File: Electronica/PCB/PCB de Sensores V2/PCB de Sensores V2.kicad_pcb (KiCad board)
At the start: 2 copper layers, 66 x 34.7 mm, 11 parts, among them J1 Conexion Sensores, U1 ULTRASONICO1, U2 ULTRASONICO2, U3 ULTRASONICO3, U4 ULTRASONICO4, U5 ULTRASONICO5

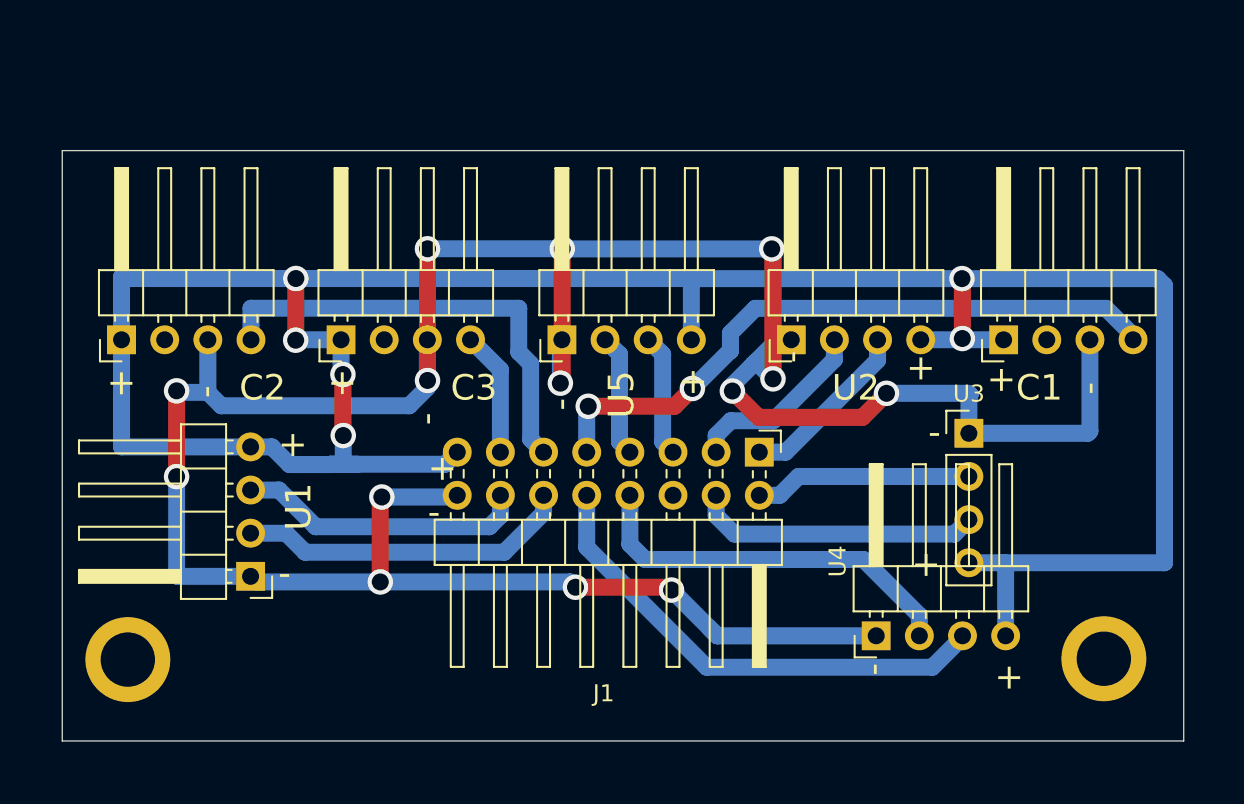
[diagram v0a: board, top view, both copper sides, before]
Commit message: PCB sensores v2 y principal v7 terminadas
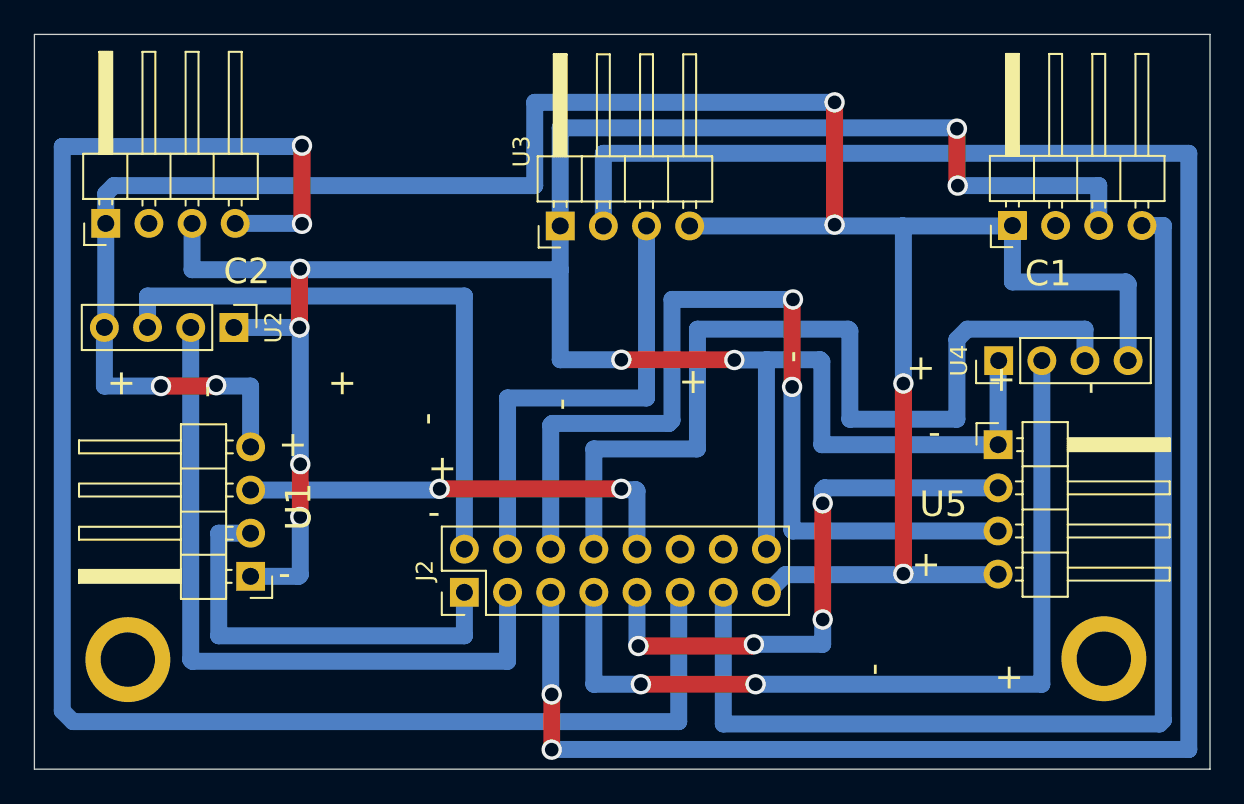
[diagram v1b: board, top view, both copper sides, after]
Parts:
- removed C3: CNY3, Connector_PinHeader_2.54mm:PinHeader_1x04_P2.54mm_Horizontal
- removed J1: Conexion Sensores, Connector_PinHeader_2.54mm:PinHeader_2x08_P2.54mm_Horizontal
- added J2: Conexion Sensores, Connector_PinHeader_2.54mm:PinHeader_2x08_P2.54mm_Vertical, F.Cu at (196.0, 68.2)
- U2, U4: footprint Connector_PinHeader_2.54mm:PinHeader_1x04_P2.54mm_Horizontal -> Connector_PinHeader_2.54mm:PinHeader_1x04_P2.54mm_Vertical
- U3: footprint Connector_PinHeader_2.54mm:PinHeader_1x04_P2.54mm_Vertical -> Connector_PinHeader_2.54mm:PinHeader_1x04_P2.54mm_Horizontal
- moved U2 32.8 mm to (182.4, 52.6), turned to -90 degrees
- moved U3 27.0 mm to (201.6, 46.7), turned to 90 degrees
- moved U5 26.4 mm to (227.4, 59.5), turned to 0 degrees
- moved U4 17.7 mm to (227.4, 54.6)
- moved C2 6.91 mm to (174.8, 46.5)
- moved C1 6.75 mm to (228.2, 46.6)
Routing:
- net ECHO 3: track 12.8 -> 120.7 mm, vias 0 -> 2
- net CNY 2: track 26.7 -> 99.7 mm, vias 0 -> 2
- net TRIG 5: track 7.22 -> 54.6 mm, vias 0 -> 2
- net ECHO 2: track 11.0 -> 42.3 mm
- net ECHO 4: track 22.9 -> 50.9 mm, vias 0 -> 2
- net ECHO 5: track 7.22 -> 33.8 mm, vias 0 -> 4
- net CNY 1: track 38.7 -> 64.1 mm, vias 2 -> 0
- net TRIG 2: track 10.4 -> 35.4 mm
- net TRIG 4: track 28.9 -> 53.9 mm
- net GND: track 168.1 -> 147.3 mm, vias 14 -> 8
- net TRIG 3: track 16.9 -> 27.2 mm
- net TRIG 1: track 17.1 -> 26.3 mm, vias 0 -> 2
- net CNY 3: track 7.34 -> 0.00 mm
- net ECHO 1: track 19.7 -> 24.9 mm
- net +5V: track 151.9 -> 147.2 mm
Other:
- board size 66 x 34.7 mm -> 69.2 x 43.3 mm
